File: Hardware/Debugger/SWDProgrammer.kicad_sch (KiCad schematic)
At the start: 37 parts, among them J1 USB_C_Receptacle_USB2.0, J2 USB_C_Receptacle_USB2.0, U1 AP2112K-3.3, U2 STM32F103C8Tx, Y1 32.768KHZ, Y2 8Mhz

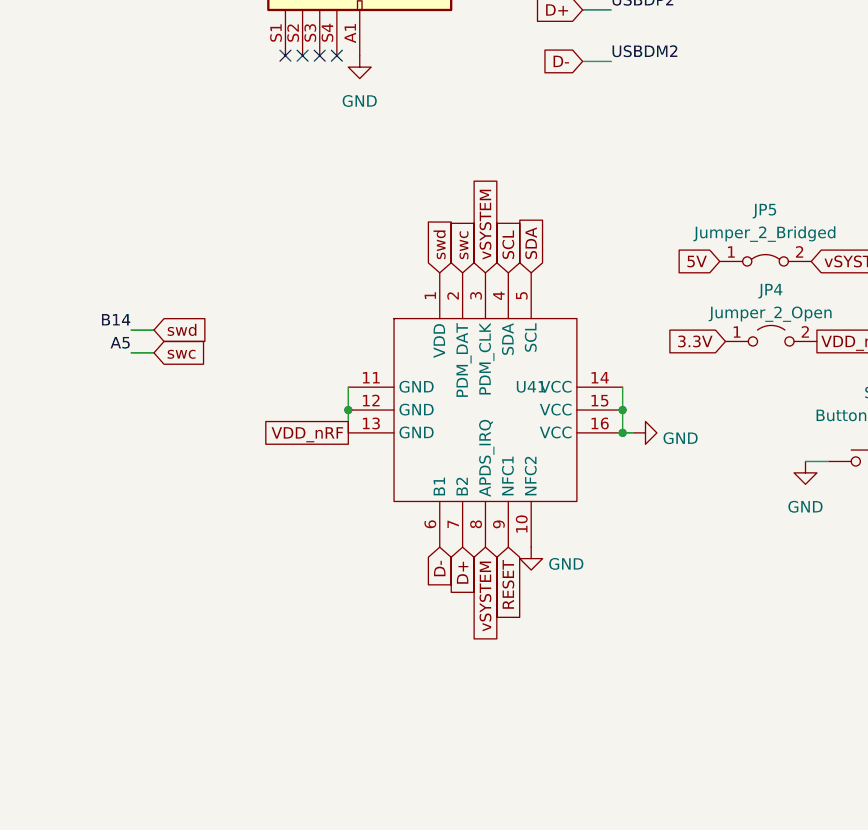
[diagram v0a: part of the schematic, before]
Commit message: new debugger
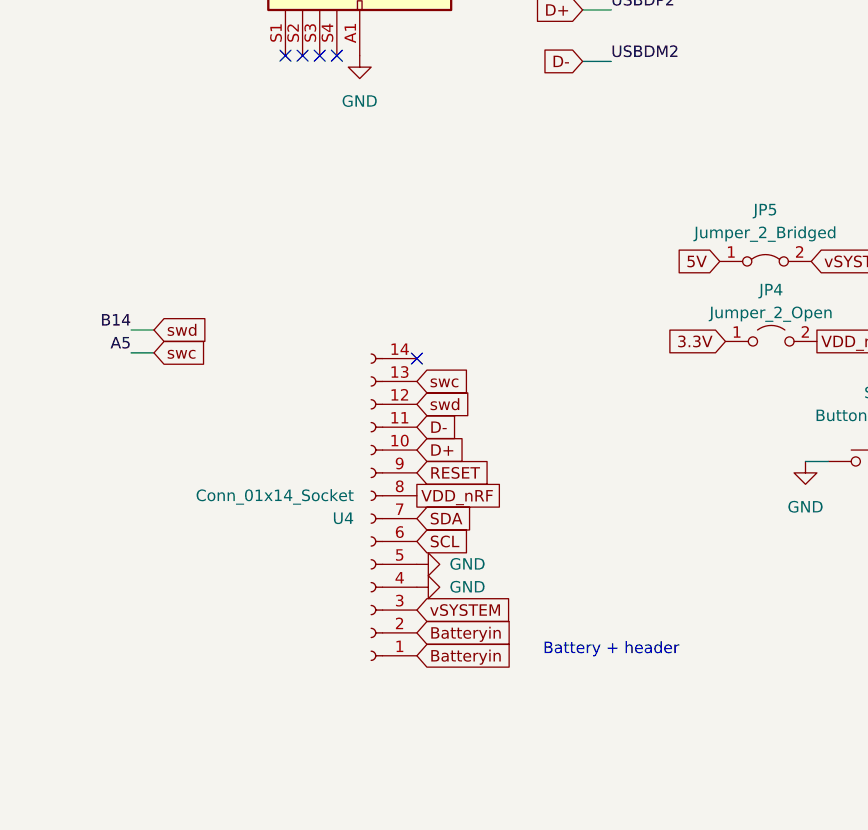
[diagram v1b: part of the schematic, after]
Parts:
- removed U41: ~, Library:BK13C06-10DP, symbol Library:BK13C06-10D(S/P)
- added U4: Conn_01x14_Socket, Library:FPC, symbol Connector:Conn_01x14_Socket
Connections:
- net 5V(2): now also U4.3 (Pin_3)
- net D+: now also U4.10 (Pin_10)
- net D-: now also U4.11 (Pin_11)
- net GND: now also U4.4 (Pin_4), U4.5 (Pin_5)
- net RESET: now also U4.9 (Pin_9)
- net SCL: now also U4.6 (Pin_6)
- net SDA: now also U4.7 (Pin_7)
- net VDD_nRF: now also U4.8 (Pin_8)
- net swc: now also U4.13 (Pin_13)
- net swd: now also U4.12 (Pin_12)
- new net Batteryin: U4.1 (Pin_1), U4.2 (Pin_2)
- no-connect marks 8 -> 9
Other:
- note added: "Battery + header"
